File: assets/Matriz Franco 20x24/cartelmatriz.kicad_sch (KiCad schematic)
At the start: 483 parts, among them J1 Conn_01x20_Socket, J2 Conn_01x24_Socket, J3 Conn_01x20_Socket

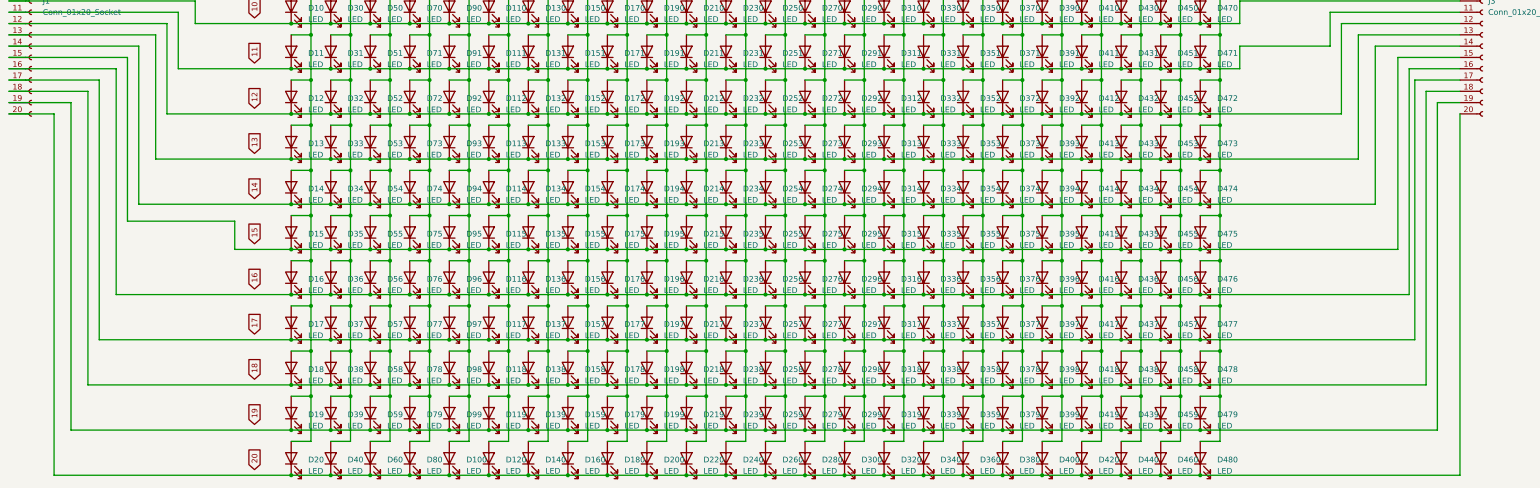
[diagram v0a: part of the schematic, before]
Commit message: finding the final
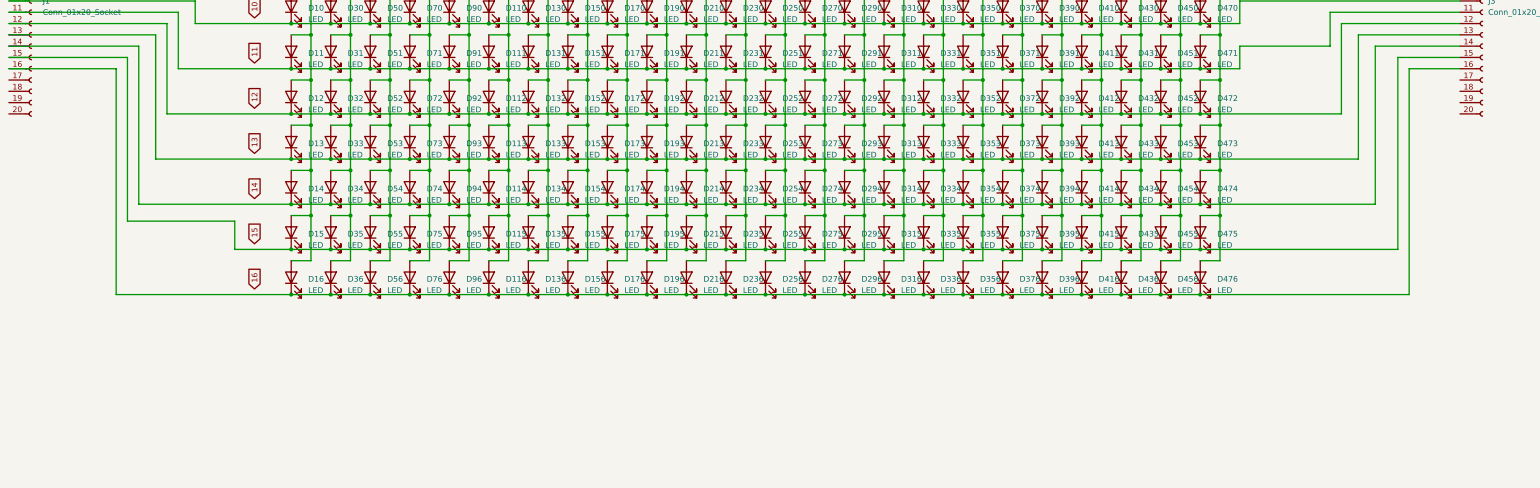
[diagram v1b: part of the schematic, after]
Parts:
- removed D100, D117, D118, D119, D120, D137, D138, D139, D140, D157, D158, D159, D160, D17, D177, D178, D179, D18, D180, D19, D197, D198, D199, D20, D200, D217, D218, D219, D220, D237, D238, D239, D240, D257, D258, D259, D260, D277, D278, D279, D280, D297, D298, D299, D300, D317, D318, D319, D320, D337, D338, D339, D340, D357, D358, D359, D360, D37, D377, D378, D379, D38, D380, D39, D397, D398, D399, D40, D400, D417, D418, D419, D420, D437, D438, D439, D440, D457, D458, D459, D460, D477, D478, D479, D480, D57, D58, D59, D60, D77, D78, D79, D80, D97, D98, D99: LED, LED_THT:LED_D5.0mm, symbol Device:LED
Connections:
- net at J3.19 (Pin_19): no longer J1.19 (Pin_19)
- net at J3.20 (Pin_20): no longer J1.20 (Pin_20)
- net at J3.17 (Pin_17): no longer J1.17 (Pin_17)
- net at J3.18 (Pin_18): no longer J1.18 (Pin_18)
